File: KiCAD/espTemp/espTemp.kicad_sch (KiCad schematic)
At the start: 7 parts, among them U1 ESP-01, U2 LD1117S33TR_SOT223, U3 DHT22,CM2303

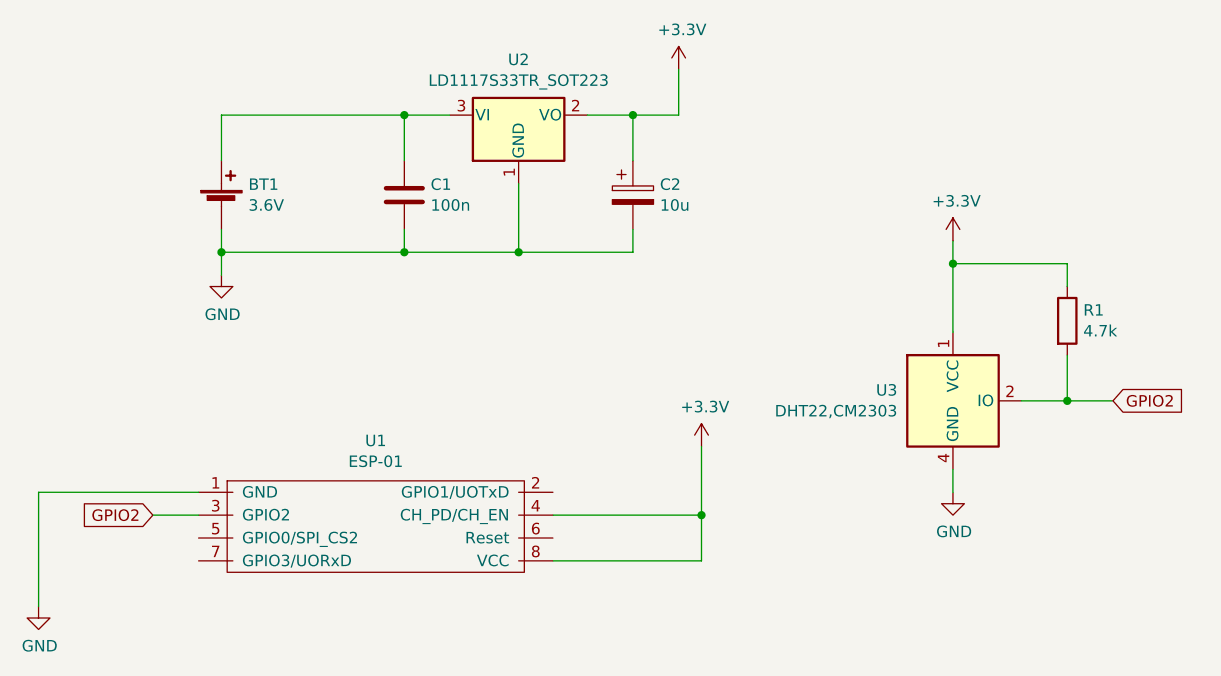
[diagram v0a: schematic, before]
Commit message: fixed kicad
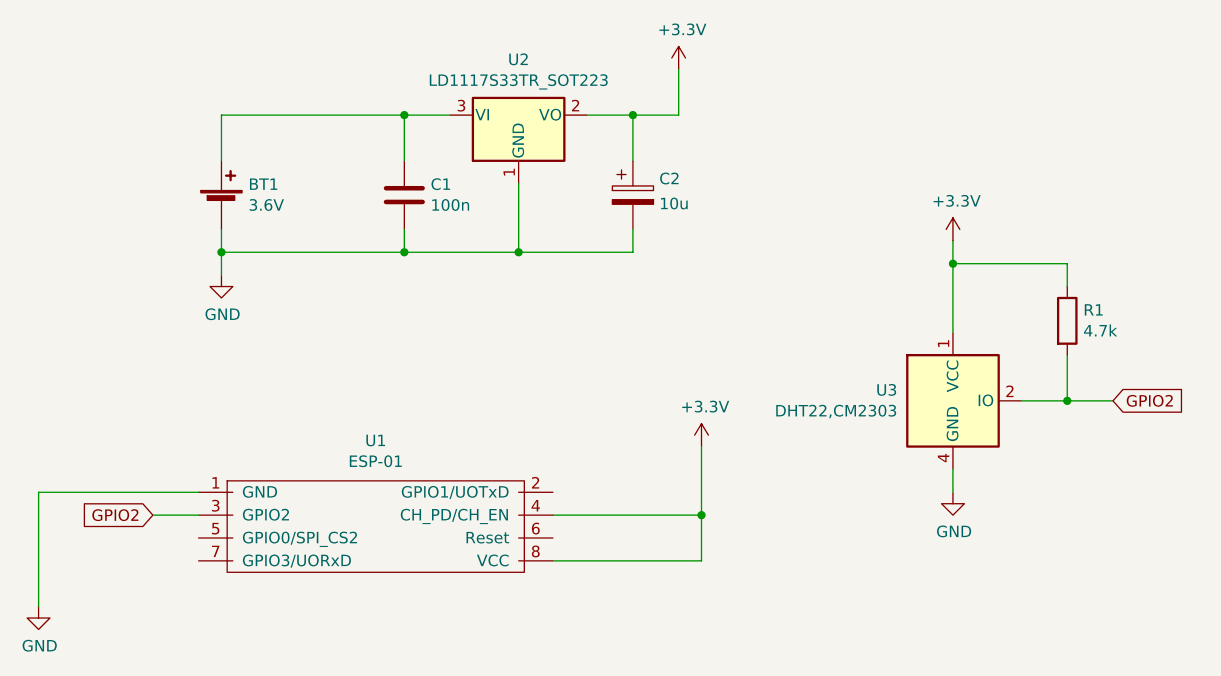
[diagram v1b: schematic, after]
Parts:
- removed C2: 10u, My_Misc:CP_Radial_D5.0mm_P2.50mm_larger_pads, symbol Device:CP
- added C2: 10u, My_Misc:CP_Radial_D5.0mm_P2.50mm_larger_pads, symbol Device:C_Polarized
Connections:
- net +3V3: now also C2.1
- net GND: now also C2.2
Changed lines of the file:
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@@
-    (pin "2")
-  )
-  (symbol (lib_id "Device:CP") (at 166.37 57.15 0) (unit 1)
-    (in_bom yes) (on_board yes)
-    (property "Reference" "C2" (id 0) (at 169.3672 55.9816 0)
-      (effects (font (size 1.27 1.27)) (justify left))
-    )
-    (property "Value" "10u" (id 1) (at 169.3672 58.293 0)
-      (effects (font (size 1.27 1.27)) (justify left))
-    )
-    (property "Footprint" "My_Misc:CP_Radial_D5.0mm_P2.50mm_larger_pads" (id 2) (at 167.3352 60.96 0)
-      (effects (font (size 1.27 1.27)) hide)
-    )
-    (property "Datasheet" "~" (id 3) (at 166.37 57.15 0)
-      (effects (font (size 1.27 1.27)) hide)
-    )
-    (pin "1")
     (pin "2")
   )
@@
     (pin "4")
   )
+  (symbol (lib_id "Device:C_Polarized") (at 166.37 57.15 0) (unit 1)
+    (in_bom yes) (on_board yes) (fields_autoplaced)
+    (property "Reference" "C2" (id 0) (at 169.291 55.3525 0)
+      (effects (font (size 1.27 1.27)) (justify left))
+    )
+    (property "Value" "10u" (id 1) (at 169.291 58.1276 0)
+      (effects (font (size 1.27 1.27)) (justify left))
+    )
+    (property "Footprint" "My_Misc:CP_Radial_D5.0mm_P2.50mm_larger_pads" (id 2) (at 167.3352 60.96 0)
+      (effects (font (size 1.27 1.27)) hide)
+    )
+    (property "Datasheet" "~" (id 3) (at 166.37 57.15 0)
+      (effects (font (size 1.27 1.27)) hide)
+    )
+    (pin "1")
+    (pin "2")
+  )
   (sheet_instances
     (path "/" (page "1"))
@@
       (reference "C1") (unit 1) (value "100n") (footprint "My_Misc:C_Disc_D3.0mm_W1.6mm_P2.50mm_larg")
     )
-    (path "/00000000-0000-0000-0000-000061a7af7d"
+    (path "/ac780ebe-5afd-4e74-82f8-509da8ddaa4d"
       (reference "C2") (unit 1) (value "10u") (footprint "My_Misc:CP_Radial_D5.0mm_P2.50mm_larger_pads")
     )
